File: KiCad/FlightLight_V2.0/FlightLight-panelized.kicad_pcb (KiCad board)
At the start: 2 copper layers, 69 x 73 mm, 116 parts, among them J3 Conn_02x05_Odd_Even, SW1 AP, U2 ULN2003, U3 ESP-12F, U4 AMS1117-3.3

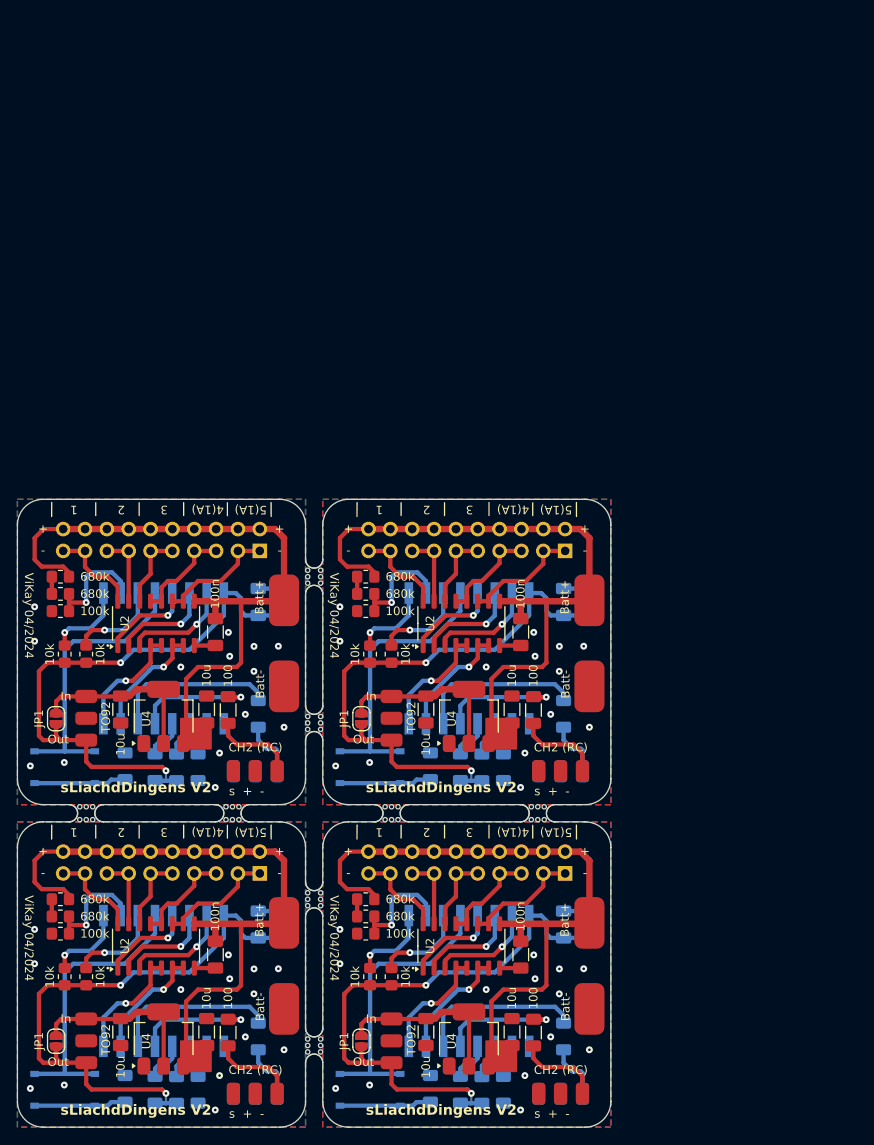
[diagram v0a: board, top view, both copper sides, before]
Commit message: new panelized
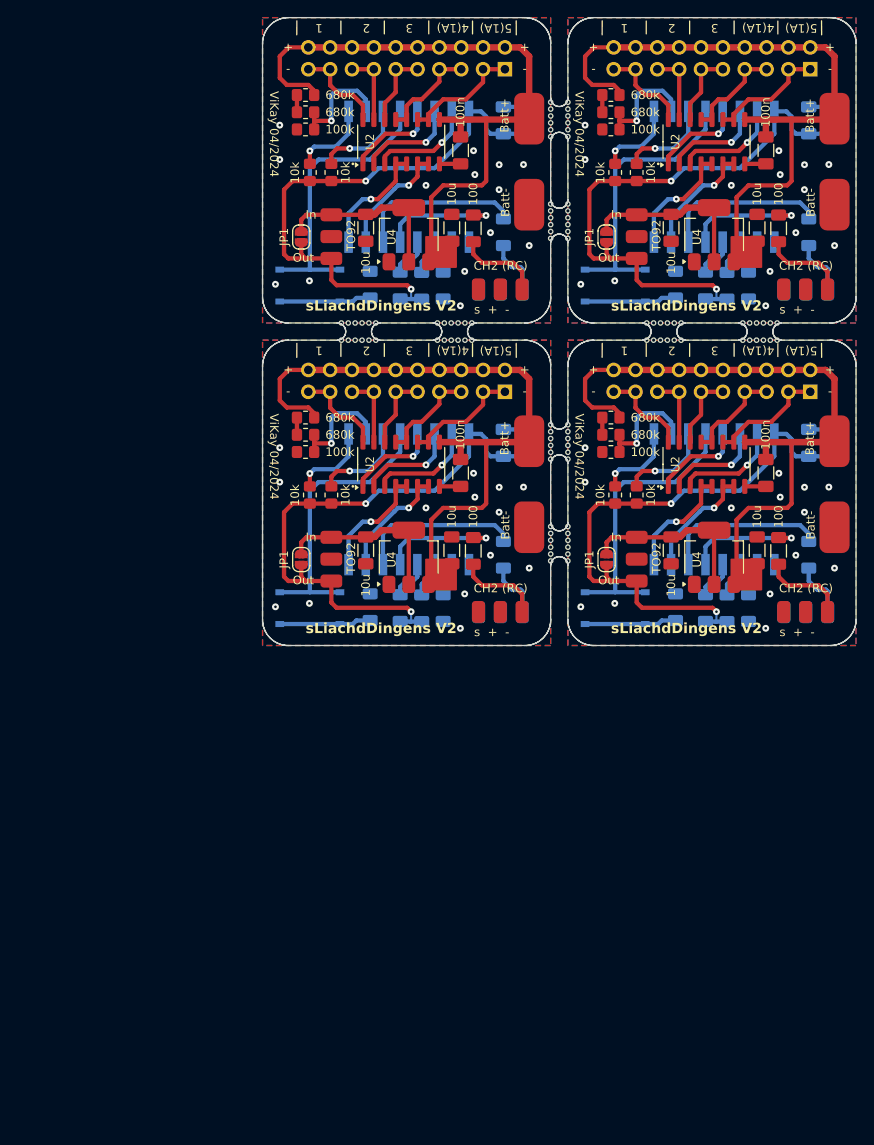
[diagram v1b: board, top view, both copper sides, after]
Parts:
- removed the Batt+1 at (152.0, 125.2)
- removed the Batt+1 at (116.5, 87.8)
- removed the Batt+1 at (116.5, 125.2)
- removed the Batt+1 at (152.0, 87.8)
- removed the Batt-1 at (116.5, 135.2)
- removed the Batt-1 at (116.5, 97.8)
- removed the Batt-1 at (152.0, 97.8)
- removed the Batt-1 at (152.0, 135.2)
- removed the C2 at (144.0, 91.4)
- removed the C2 at (144.0, 128.9)
- removed the C2 at (108.5, 128.9)
- removed the C2 at (108.5, 91.4)
- removed the C3 at (143.0, 100.4)
- removed the C3 at (107.5, 137.9)
- removed the C3 at (107.5, 100.4)
- removed the C3 at (143.0, 137.9)
- removed the C4 at (97.5, 137.9)
- removed the C4 at (133.0, 137.9)
- removed the C4 at (97.5, 100.4)
- removed the C4 at (133.0, 100.4)
- removed the C5 at (113.5, 87.9)
- removed the C5 at (149.0, 125.4)
- removed the C5 at (149.0, 87.9)
- removed the C5 at (113.5, 125.4)
- removed the C6 at (116.0, 87.9)
- removed the C6 at (151.5, 125.4)
- removed the C6 at (116.0, 125.4)
- removed the C6 at (151.5, 87.9)
- removed the CH1(RC)1 at (151.2, 107.6)
- removed the CH1(RC)1 at (115.7, 107.6)
- removed the CH1(RC)1 at (115.7, 145.1)
- removed the CH1(RC)1 at (151.2, 145.1)
- removed the CH2(RC)1 at (115.7, 145.1)
- removed the CH2(RC)1 at (115.7, 107.6)
- removed the CH2(RC)1 at (151.2, 145.1)
- removed the CH2(RC)1 at (151.2, 107.6)
- removed the J3 at (113.7, 82.0)
- removed the J3 at (149.2, 119.5)
- removed the J3 at (149.2, 82.0)
- removed the J3 at (113.7, 119.5)
- removed the JP1 at (125.5, 101.5)
- removed the JP1 at (90.0, 139.0)
- removed the JP1 at (90.0, 101.5)
- removed the JP1 at (125.5, 139.0)
- removed the R1 at (129.0, 94.0)
- removed the R1 at (129.0, 131.5)
- removed the R1 at (93.5, 131.5)
- removed the R1 at (93.5, 94.0)
- removed the R10 at (90.5, 124.5)
- removed the R10 at (126.0, 124.5)
- removed the R10 at (90.5, 87.0)
- removed the R10 at (126.0, 87.0)
- removed the R11 at (90.5, 122.5)
- removed the R11 at (126.0, 85.0)
- removed the R11 at (90.5, 85.0)
- removed the R11 at (126.0, 122.5)
- removed the R2 at (133.5, 144.5)
- removed the R2 at (98.0, 144.5)
- removed the R2 at (98.0, 107.0)
- removed the R2 at (133.5, 107.0)
- removed the R3 at (126.5, 94.0)
- removed the R3 at (91.0, 94.0)
- removed the R3 at (91.0, 131.5)
- removed the R3 at (126.5, 131.5)
- removed the R4 at (137.0, 144.6)
- removed the R4 at (101.5, 144.6)
- removed the R4 at (137.0, 107.1)
- removed the R4 at (101.5, 107.1)
- removed the R5 at (104.0, 144.7)
- removed the R5 at (104.0, 107.2)
- removed the R5 at (139.5, 144.7)
- removed the R5 at (139.5, 107.2)
- removed the R6 at (106.5, 144.7)
- removed the R6 at (142.0, 144.7)
- removed the R6 at (142.0, 107.2)
- removed the R6 at (106.5, 107.2)
- removed the R7 at (149.0, 138.4)
- removed the R7 at (113.5, 101.0)
- removed the R7 at (149.0, 101.0)
- removed the R7 at (113.5, 138.4)
- removed the R8 at (145.5, 100.5)
- removed the R8 at (110.0, 138.0)
- removed the R8 at (110.0, 100.5)
- removed the R8 at (145.5, 138.0)
- removed the R9 at (90.5, 89.0)
- removed the R9 at (126.0, 89.0)
- removed the R9 at (90.5, 126.5)
- removed the R9 at (126.0, 126.5)
- removed the SW1 at (91.0, 144.7)
- removed the SW1 at (91.0, 107.2)
- removed the SW1 at (126.5, 107.2)
- removed the SW1 at (126.5, 144.7)
- removed the TO92 at (129.0, 136.4)
- removed the TO92 at (93.5, 98.9)
- removed the TO92 at (129.0, 98.9)
- removed the TO92 at (93.5, 136.4)
- removed the U2 at (137.1, 127.9)
- removed the U2 at (101.6, 90.4)
- removed the U2 at (137.1, 90.4)
- removed the U2 at (101.6, 127.9)
- removed the U3 at (134.5, 94.5)
- removed the U3 at (99.0, 132.0)
- removed the U3 at (134.5, 132.0)
- removed the U3 at (99.0, 94.5)
- removed the U4 at (138.0, 101.2)
- removed the U4 at (138.0, 138.7)
- removed the U4 at (102.5, 101.2)
- removed the U4 at (102.5, 138.7)
- removed mouse-bite-2mm-slot (x8): VAL**, Panelization:mouse-bite-2mm-slot
- added Batt+1: Batt+, ViKay:Conn_01x01_2.54_big, F.Cu at (145.0, 69.2)
- added Batt+1: Batt+, ViKay:Conn_01x01_2.54_big, F.Cu at (180.5, 69.2)
- added Batt+1: Batt+, ViKay:Conn_01x01_2.54_big, F.Cu at (180.5, 31.8)
- added Batt+1: Batt+, ViKay:Conn_01x01_2.54_big, F.Cu at (145.0, 31.8)
- added Batt-1: Batt-, ViKay:Conn_01x01_2.54_big, F.Cu at (180.5, 79.2)
- added Batt-1: Batt-, ViKay:Conn_01x01_2.54_big, F.Cu at (145.0, 79.2)
- added Batt-1: Batt-, ViKay:Conn_01x01_2.54_big, F.Cu at (145.0, 41.8)
- added Batt-1: Batt-, ViKay:Conn_01x01_2.54_big, F.Cu at (180.5, 41.8)
- added C2: 100n, Capacitor_SMD:C_1206_3216Metric_Pad1.33x1.80mm_HandSolder, F.Cu at (137.0, 72.9)
- added C2: 100n, Capacitor_SMD:C_1206_3216Metric_Pad1.33x1.80mm_HandSolder, F.Cu at (137.0, 35.4)
- added C2: 100n, Capacitor_SMD:C_1206_3216Metric_Pad1.33x1.80mm_HandSolder, F.Cu at (172.5, 72.9)
- added C2: 100n, Capacitor_SMD:C_1206_3216Metric_Pad1.33x1.80mm_HandSolder, F.Cu at (172.5, 35.4)
- added C3: 10u, Capacitor_SMD:C_1206_3216Metric_Pad1.33x1.80mm_HandSolder, F.Cu at (171.5, 44.4)
- added C3: 10u, Capacitor_SMD:C_1206_3216Metric_Pad1.33x1.80mm_HandSolder, F.Cu at (171.5, 81.9)
- added C3: 10u, Capacitor_SMD:C_1206_3216Metric_Pad1.33x1.80mm_HandSolder, F.Cu at (136.0, 44.4)
- added C3: 10u, Capacitor_SMD:C_1206_3216Metric_Pad1.33x1.80mm_HandSolder, F.Cu at (136.0, 81.9)
- added C4: 10u, Capacitor_SMD:C_1206_3216Metric_Pad1.33x1.80mm_HandSolder, F.Cu at (161.5, 81.9)
- added C4: 10u, Capacitor_SMD:C_1206_3216Metric_Pad1.33x1.80mm_HandSolder, F.Cu at (126.0, 44.4)
- added C4: 10u, Capacitor_SMD:C_1206_3216Metric_Pad1.33x1.80mm_HandSolder, F.Cu at (161.5, 44.4)
- added C4: 10u, Capacitor_SMD:C_1206_3216Metric_Pad1.33x1.80mm_HandSolder, F.Cu at (126.0, 81.9)
- added C5: 100n, Capacitor_SMD:C_1206_3216Metric_Pad1.33x1.80mm_HandSolder, B.Cu at (142.0, 31.9)
- added C5: 100n, Capacitor_SMD:C_1206_3216Metric_Pad1.33x1.80mm_HandSolder, B.Cu at (142.0, 69.4)
- added C5: 100n, Capacitor_SMD:C_1206_3216Metric_Pad1.33x1.80mm_HandSolder, B.Cu at (177.5, 69.4)
- added C5: 100n, Capacitor_SMD:C_1206_3216Metric_Pad1.33x1.80mm_HandSolder, B.Cu at (177.5, 31.9)
- added C6: 10u, Capacitor_SMD:C_1206_3216Metric_Pad1.33x1.80mm_HandSolder, B.Cu at (144.5, 69.4)
- added C6: 10u, Capacitor_SMD:C_1206_3216Metric_Pad1.33x1.80mm_HandSolder, B.Cu at (180.0, 69.4)
- added C6: 10u, Capacitor_SMD:C_1206_3216Metric_Pad1.33x1.80mm_HandSolder, B.Cu at (180.0, 31.9)
- added C6: 10u, Capacitor_SMD:C_1206_3216Metric_Pad1.33x1.80mm_HandSolder, B.Cu at (144.5, 31.9)
- added CH1(RC)1: CH1 (RC), ViKay:Conn_01x03_2.54_small, B.Cu at (144.2, 89.1)
- added CH1(RC)1: CH1 (RC), ViKay:Conn_01x03_2.54_small, B.Cu at (179.7, 89.1)
- added CH1(RC)1: CH1 (RC), ViKay:Conn_01x03_2.54_small, B.Cu at (179.7, 51.6)
- added CH1(RC)1: CH1 (RC), ViKay:Conn_01x03_2.54_small, B.Cu at (144.2, 51.6)
- added CH2(RC)1: CH2 (RC) LowPower, ViKay:Conn_01x03_2.54_small, F.Cu at (179.7, 51.6)
- added CH2(RC)1: CH2 (RC) LowPower, ViKay:Conn_01x03_2.54_small, F.Cu at (144.2, 89.1)
- added CH2(RC)1: CH2 (RC) LowPower, ViKay:Conn_01x03_2.54_small, F.Cu at (144.2, 51.6)
- added CH2(RC)1: CH2 (RC) LowPower, ViKay:Conn_01x03_2.54_small, F.Cu at (179.7, 89.1)
- added J3: Conn_02x05_Odd_Even, Connector_PinHeader_2.54mm:PinHeader_2x10_P2.54mm_Vertical, B.Cu at (177.7, 63.5)
- added J3: Conn_02x05_Odd_Even, Connector_PinHeader_2.54mm:PinHeader_2x10_P2.54mm_Vertical, B.Cu at (177.7, 26.0)
- added J3: Conn_02x05_Odd_Even, Connector_PinHeader_2.54mm:PinHeader_2x10_P2.54mm_Vertical, B.Cu at (142.2, 26.0)
- added J3: Conn_02x05_Odd_Even, Connector_PinHeader_2.54mm:PinHeader_2x10_P2.54mm_Vertical, B.Cu at (142.2, 63.5)
- added JP1: kein Supervisor, Jumper:SolderJumper-2_P1.3mm_Open_RoundedPad1.0x1.5mm, F.Cu at (118.5, 45.5)
- added JP1: kein Supervisor, Jumper:SolderJumper-2_P1.3mm_Open_RoundedPad1.0x1.5mm, F.Cu at (118.5, 83.0)
- added JP1: kein Supervisor, Jumper:SolderJumper-2_P1.3mm_Open_RoundedPad1.0x1.5mm, F.Cu at (154.0, 83.0)
- added JP1: kein Supervisor, Jumper:SolderJumper-2_P1.3mm_Open_RoundedPad1.0x1.5mm, F.Cu at (154.0, 45.5)
- added KiKit_MB_10_1: NPTH, NPTH, F.Cu at (147.5, 79.2)
- added KiKit_MB_10_2: NPTH, NPTH, F.Cu at (147.5, 80.0)
- added KiKit_MB_10_3: NPTH, NPTH, F.Cu at (147.5, 80.8)
- added KiKit_MB_10_4: NPTH, NPTH, F.Cu at (147.5, 81.6)
- added KiKit_MB_10_5: NPTH, NPTH, F.Cu at (147.5, 82.4)
- added KiKit_MB_10_6: NPTH, NPTH, F.Cu at (147.5, 83.2)
- added KiKit_MB_11_1: NPTH, NPTH, F.Cu at (123.2, 57.5)
- added KiKit_MB_11_2: NPTH, NPTH, F.Cu at (124.0, 57.5)
- added KiKit_MB_11_3: NPTH, NPTH, F.Cu at (124.8, 57.5)
- added KiKit_MB_11_4: NPTH, NPTH, F.Cu at (125.6, 57.5)
- added KiKit_MB_11_5: NPTH, NPTH, F.Cu at (126.4, 57.5)
- added KiKit_MB_11_6: NPTH, NPTH, F.Cu at (127.2, 57.5)
- added KiKit_MB_12_1: NPTH, NPTH, F.Cu at (134.3, 57.5)
- added KiKit_MB_12_2: NPTH, NPTH, F.Cu at (135.1, 57.5)
- added KiKit_MB_12_3: NPTH, NPTH, F.Cu at (135.9, 57.5)
- added KiKit_MB_12_4: NPTH, NPTH, F.Cu at (136.7, 57.5)
- added KiKit_MB_12_5: NPTH, NPTH, F.Cu at (137.5, 57.5)
- added KiKit_MB_12_6: NPTH, NPTH, F.Cu at (138.3, 57.5)
- added KiKit_MB_13_1: NPTH, NPTH, F.Cu at (149.5, 71.3)
- added KiKit_MB_13_2: NPTH, NPTH, F.Cu at (149.5, 70.5)
- added KiKit_MB_13_3: NPTH, NPTH, F.Cu at (149.5, 69.7)
- added KiKit_MB_13_4: NPTH, NPTH, F.Cu at (149.5, 68.9)
- added KiKit_MB_13_5: NPTH, NPTH, F.Cu at (149.5, 68.1)
- added KiKit_MB_13_6: NPTH, NPTH, F.Cu at (149.5, 67.3)
- added KiKit_MB_14_1: NPTH, NPTH, F.Cu at (149.5, 83.2)
- added KiKit_MB_14_2: NPTH, NPTH, F.Cu at (149.5, 82.4)
- added KiKit_MB_14_3: NPTH, NPTH, F.Cu at (149.5, 81.6)
- added KiKit_MB_14_4: NPTH, NPTH, F.Cu at (149.5, 80.8)
- added KiKit_MB_14_5: NPTH, NPTH, F.Cu at (149.5, 80.0)
- added KiKit_MB_14_6: NPTH, NPTH, F.Cu at (149.5, 79.2)
- added KiKit_MB_15_1: NPTH, NPTH, F.Cu at (158.7, 57.5)
- added KiKit_MB_15_2: NPTH, NPTH, F.Cu at (159.5, 57.5)
- added KiKit_MB_15_3: NPTH, NPTH, F.Cu at (160.3, 57.5)
- added KiKit_MB_15_4: NPTH, NPTH, F.Cu at (161.1, 57.5)
- added KiKit_MB_15_5: NPTH, NPTH, F.Cu at (161.9, 57.5)
- added KiKit_MB_15_6: NPTH, NPTH, F.Cu at (162.7, 57.5)
- added KiKit_MB_16_1: NPTH, NPTH, F.Cu at (169.8, 57.5)
- added KiKit_MB_16_2: NPTH, NPTH, F.Cu at (170.6, 57.5)
- added KiKit_MB_16_3: NPTH, NPTH, F.Cu at (171.4, 57.5)
- added KiKit_MB_16_4: NPTH, NPTH, F.Cu at (172.2, 57.5)
- added KiKit_MB_16_5: NPTH, NPTH, F.Cu at (173.0, 57.5)
- added KiKit_MB_16_6: NPTH, NPTH, F.Cu at (173.8, 57.5)
- added KiKit_MB_1_1: NPTH, NPTH, F.Cu at (147.5, 29.8)
- added KiKit_MB_1_2: NPTH, NPTH, F.Cu at (147.5, 30.6)
- added KiKit_MB_1_3: NPTH, NPTH, F.Cu at (147.5, 31.4)
- added KiKit_MB_1_4: NPTH, NPTH, F.Cu at (147.5, 32.2)
- added KiKit_MB_1_5: NPTH, NPTH, F.Cu at (147.5, 33.0)
- added KiKit_MB_1_6: NPTH, NPTH, F.Cu at (147.5, 33.8)
- added KiKit_MB_2_1: NPTH, NPTH, F.Cu at (147.5, 41.7)
- added KiKit_MB_2_2: NPTH, NPTH, F.Cu at (147.5, 42.5)
- added KiKit_MB_2_3: NPTH, NPTH, F.Cu at (147.5, 43.3)
- added KiKit_MB_2_4: NPTH, NPTH, F.Cu at (147.5, 44.1)
- added KiKit_MB_2_5: NPTH, NPTH, F.Cu at (147.5, 44.9)
- added KiKit_MB_2_6: NPTH, NPTH, F.Cu at (147.5, 45.7)
- added KiKit_MB_3_1: NPTH, NPTH, F.Cu at (127.2, 55.5)
- added KiKit_MB_3_2: NPTH, NPTH, F.Cu at (126.4, 55.5)
- added KiKit_MB_3_3: NPTH, NPTH, F.Cu at (125.6, 55.5)
- added KiKit_MB_3_4: NPTH, NPTH, F.Cu at (124.8, 55.5)
- added KiKit_MB_3_5: NPTH, NPTH, F.Cu at (124.0, 55.5)
- added KiKit_MB_3_6: NPTH, NPTH, F.Cu at (123.2, 55.5)
- added KiKit_MB_4_1: NPTH, NPTH, F.Cu at (138.3, 55.5)
- added KiKit_MB_4_2: NPTH, NPTH, F.Cu at (137.5, 55.5)
- added KiKit_MB_4_3: NPTH, NPTH, F.Cu at (136.7, 55.5)
- added KiKit_MB_4_4: NPTH, NPTH, F.Cu at (135.9, 55.5)
- added KiKit_MB_4_5: NPTH, NPTH, F.Cu at (135.1, 55.5)
- added KiKit_MB_4_6: NPTH, NPTH, F.Cu at (134.3, 55.5)
- added KiKit_MB_5_1: NPTH, NPTH, F.Cu at (149.5, 33.8)
- added KiKit_MB_5_2: NPTH, NPTH, F.Cu at (149.5, 33.0)
- added KiKit_MB_5_3: NPTH, NPTH, F.Cu at (149.5, 32.2)
- added KiKit_MB_5_4: NPTH, NPTH, F.Cu at (149.5, 31.4)
- added KiKit_MB_5_5: NPTH, NPTH, F.Cu at (149.5, 30.6)
- added KiKit_MB_5_6: NPTH, NPTH, F.Cu at (149.5, 29.8)
- added KiKit_MB_6_1: NPTH, NPTH, F.Cu at (149.5, 45.7)
- added KiKit_MB_6_2: NPTH, NPTH, F.Cu at (149.5, 44.9)
- added KiKit_MB_6_3: NPTH, NPTH, F.Cu at (149.5, 44.1)
- added KiKit_MB_6_4: NPTH, NPTH, F.Cu at (149.5, 43.3)
- added KiKit_MB_6_5: NPTH, NPTH, F.Cu at (149.5, 42.5)
- added KiKit_MB_6_6: NPTH, NPTH, F.Cu at (149.5, 41.7)
- added KiKit_MB_7_1: NPTH, NPTH, F.Cu at (162.7, 55.5)
- added KiKit_MB_7_2: NPTH, NPTH, F.Cu at (161.9, 55.5)
- added KiKit_MB_7_3: NPTH, NPTH, F.Cu at (161.1, 55.5)
- added KiKit_MB_7_4: NPTH, NPTH, F.Cu at (160.3, 55.5)
- added KiKit_MB_7_5: NPTH, NPTH, F.Cu at (159.5, 55.5)
- added KiKit_MB_7_6: NPTH, NPTH, F.Cu at (158.7, 55.5)
- added KiKit_MB_8_1: NPTH, NPTH, F.Cu at (173.8, 55.5)
- added KiKit_MB_8_2: NPTH, NPTH, F.Cu at (173.0, 55.5)
- added KiKit_MB_8_3: NPTH, NPTH, F.Cu at (172.2, 55.5)
- added KiKit_MB_8_4: NPTH, NPTH, F.Cu at (171.4, 55.5)
- added KiKit_MB_8_5: NPTH, NPTH, F.Cu at (170.6, 55.5)
- added KiKit_MB_8_6: NPTH, NPTH, F.Cu at (169.8, 55.5)
- added KiKit_MB_9_1: NPTH, NPTH, F.Cu at (147.5, 67.3)
- added KiKit_MB_9_2: NPTH, NPTH, F.Cu at (147.5, 68.1)
- added KiKit_MB_9_3: NPTH, NPTH, F.Cu at (147.5, 68.9)
- added KiKit_MB_9_4: NPTH, NPTH, F.Cu at (147.5, 69.7)
- added KiKit_MB_9_5: NPTH, NPTH, F.Cu at (147.5, 70.5)
- added KiKit_MB_9_6: NPTH, NPTH, F.Cu at (147.5, 71.3)
- added R1: 10k, Resistor_SMD:R_0805_2012Metric_Pad1.20x1.40mm_HandSolder, F.Cu at (157.5, 38.0)
- added R1: 10k, Resistor_SMD:R_0805_2012Metric_Pad1.20x1.40mm_HandSolder, F.Cu at (157.5, 75.5)
- added R1: 10k, Resistor_SMD:R_0805_2012Metric_Pad1.20x1.40mm_HandSolder, F.Cu at (122.0, 75.5)
- added R1: 10k, Resistor_SMD:R_0805_2012Metric_Pad1.20x1.40mm_HandSolder, F.Cu at (122.0, 38.0)
- added R10: 680k, Resistor_SMD:R_0805_2012Metric_Pad1.20x1.40mm_HandSolder, F.Cu at (154.5, 31.0)
- added R10: 680k, Resistor_SMD:R_0805_2012Metric_Pad1.20x1.40mm_HandSolder, F.Cu at (154.5, 68.5)
- added R10: 680k, Resistor_SMD:R_0805_2012Metric_Pad1.20x1.40mm_HandSolder, F.Cu at (119.0, 68.5)
- added R10: 680k, Resistor_SMD:R_0805_2012Metric_Pad1.20x1.40mm_HandSolder, F.Cu at (119.0, 31.0)
- added R11: 680k, Resistor_SMD:R_0805_2012Metric_Pad1.20x1.40mm_HandSolder, F.Cu at (154.5, 29.0)
- added R11: 680k, Resistor_SMD:R_0805_2012Metric_Pad1.20x1.40mm_HandSolder, F.Cu at (119.0, 29.0)
- added R11: 680k, Resistor_SMD:R_0805_2012Metric_Pad1.20x1.40mm_HandSolder, F.Cu at (154.5, 66.5)
- added R11: 680k, Resistor_SMD:R_0805_2012Metric_Pad1.20x1.40mm_HandSolder, F.Cu at (119.0, 66.5)
- added R2: 10k, Resistor_SMD:R_1206_3216Metric_Pad1.30x1.75mm_HandSolder, B.Cu at (126.5, 51.0)
- added R2: 10k, Resistor_SMD:R_1206_3216Metric_Pad1.30x1.75mm_HandSolder, B.Cu at (126.5, 88.5)
- added R2: 10k, Resistor_SMD:R_1206_3216Metric_Pad1.30x1.75mm_HandSolder, B.Cu at (162.0, 88.5)
- added R2: 10k, Resistor_SMD:R_1206_3216Metric_Pad1.30x1.75mm_HandSolder, B.Cu at (162.0, 51.0)
- added R3: 10k, Resistor_SMD:R_0805_2012Metric_Pad1.20x1.40mm_HandSolder, F.Cu at (155.0, 75.5)
- added R3: 10k, Resistor_SMD:R_0805_2012Metric_Pad1.20x1.40mm_HandSolder, F.Cu at (119.5, 38.0)
- added R3: 10k, Resistor_SMD:R_0805_2012Metric_Pad1.20x1.40mm_HandSolder, F.Cu at (119.5, 75.5)
- added R3: 10k, Resistor_SMD:R_0805_2012Metric_Pad1.20x1.40mm_HandSolder, F.Cu at (155.0, 38.0)
- added R4: 10k, Resistor_SMD:R_1206_3216Metric_Pad1.30x1.75mm_HandSolder, B.Cu at (130.0, 51.1)
- added R4: 10k, Resistor_SMD:R_1206_3216Metric_Pad1.30x1.75mm_HandSolder, B.Cu at (130.0, 88.6)
- added R4: 10k, Resistor_SMD:R_1206_3216Metric_Pad1.30x1.75mm_HandSolder, B.Cu at (165.5, 88.6)
- added R4: 10k, Resistor_SMD:R_1206_3216Metric_Pad1.30x1.75mm_HandSolder, B.Cu at (165.5, 51.1)
- added R5: 10k, Resistor_SMD:R_1206_3216Metric_Pad1.30x1.75mm_HandSolder, B.Cu at (132.5, 88.7)
- added R5: 10k, Resistor_SMD:R_1206_3216Metric_Pad1.30x1.75mm_HandSolder, B.Cu at (168.0, 51.2)
- added R5: 10k, Resistor_SMD:R_1206_3216Metric_Pad1.30x1.75mm_HandSolder, B.Cu at (168.0, 88.7)
- added R5: 10k, Resistor_SMD:R_1206_3216Metric_Pad1.30x1.75mm_HandSolder, B.Cu at (132.5, 51.2)
- added R6: 10k, Resistor_SMD:R_1206_3216Metric_Pad1.30x1.75mm_HandSolder, B.Cu at (170.5, 51.1)
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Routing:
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- added copper zone on B.Cu, net Board_0--BATT
- added copper zone on F.Cu, net Board_0--BATT
- added copper zone on B.Cu, net Board_1--BATT
- added copper zone on F.Cu, net Board_1--BATT
- added copper zone on B.Cu, net Board_2--BATT
- added copper zone on F.Cu, net Board_2--BATT
- added copper zone on B.Cu, net Board_3--BATT
- added copper zone on F.Cu, net Board_3--BATT
- removed copper zone on B.Cu, net -BATT
- removed copper zone on F.Cu, net -BATT
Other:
- outline, holes or cut-outs redrawn

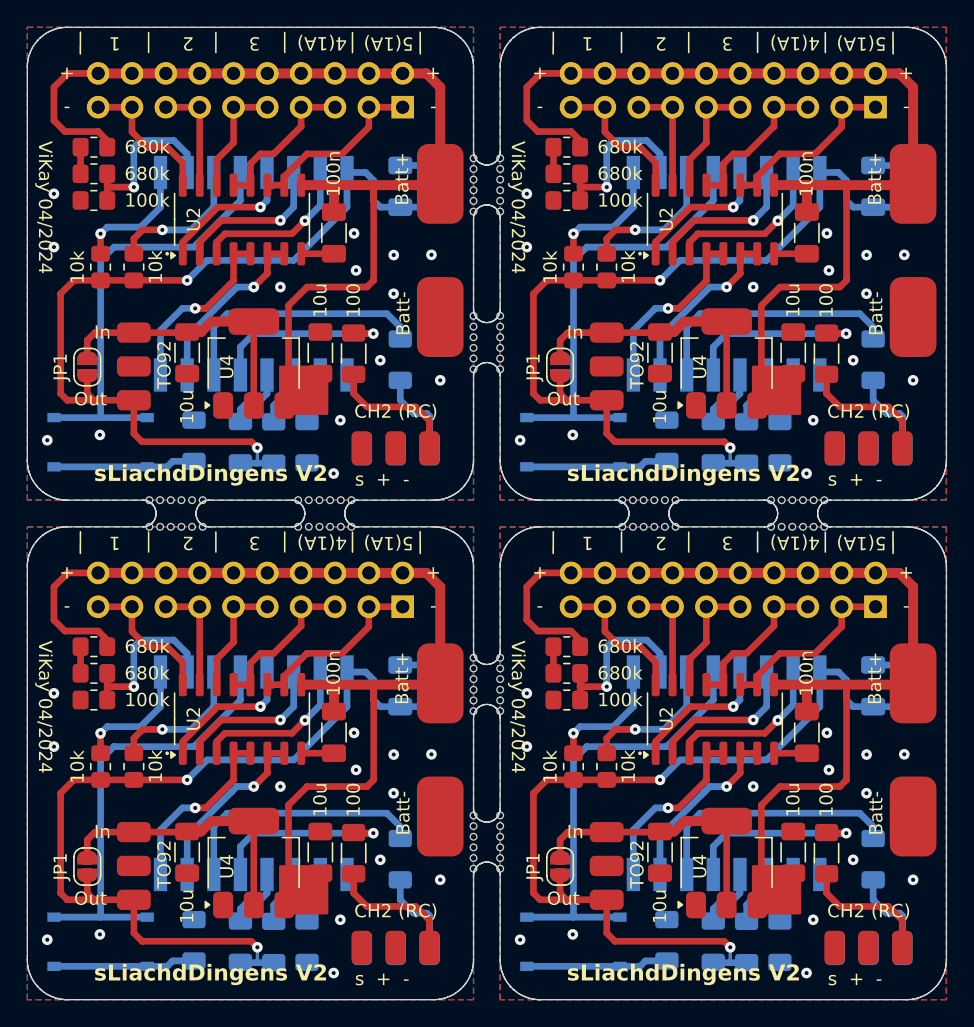
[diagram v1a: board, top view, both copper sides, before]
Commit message: PCB V2.1
kleine Fixes
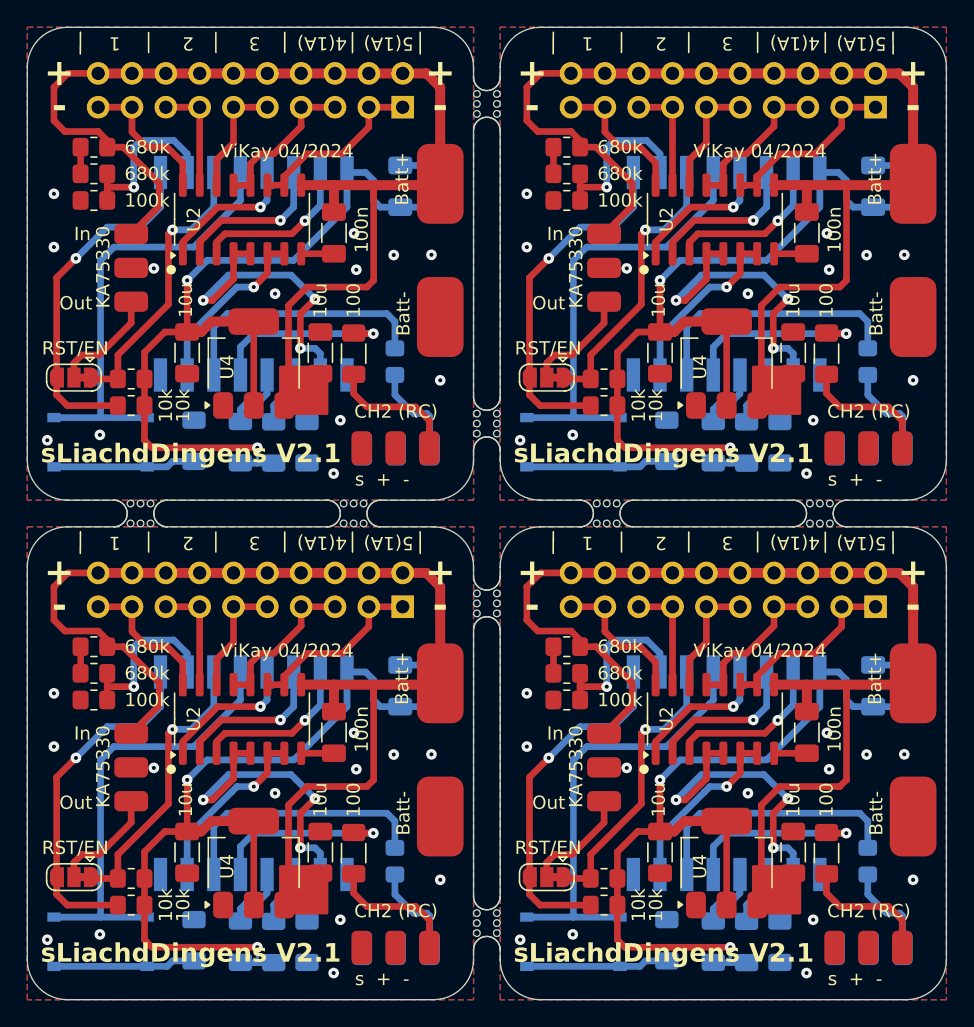
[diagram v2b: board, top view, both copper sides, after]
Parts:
- removed the JP1 at (118.5, 45.5)
- removed the JP1 at (118.5, 83.0)
- removed the JP1 at (154.0, 83.0)
- removed the JP1 at (154.0, 45.5)
- removed KiKit_MB_10_1, KiKit_MB_10_2, KiKit_MB_10_3, KiKit_MB_10_4, KiKit_MB_10_5, KiKit_MB_10_6, KiKit_MB_11_1, KiKit_MB_11_2, KiKit_MB_11_3, KiKit_MB_11_4, KiKit_MB_11_5, KiKit_MB_11_6, KiKit_MB_12_1, KiKit_MB_12_2, KiKit_MB_12_3, KiKit_MB_12_4, KiKit_MB_12_5, KiKit_MB_12_6, KiKit_MB_13_1, KiKit_MB_13_2, KiKit_MB_13_3, KiKit_MB_13_4, KiKit_MB_13_5, KiKit_MB_13_6, KiKit_MB_14_1, KiKit_MB_14_2, KiKit_MB_14_3, KiKit_MB_14_4, KiKit_MB_14_5, KiKit_MB_14_6, KiKit_MB_15_1, KiKit_MB_15_2, KiKit_MB_15_3, KiKit_MB_15_4, KiKit_MB_15_5, KiKit_MB_15_6, KiKit_MB_16_1, KiKit_MB_16_2, KiKit_MB_16_3, KiKit_MB_16_4, KiKit_MB_16_5, KiKit_MB_16_6, KiKit_MB_1_1, KiKit_MB_1_2, KiKit_MB_1_3, KiKit_MB_1_4, KiKit_MB_1_5, KiKit_MB_1_6, KiKit_MB_2_1, KiKit_MB_2_2, KiKit_MB_2_3, KiKit_MB_2_4, KiKit_MB_2_5, KiKit_MB_2_6, KiKit_MB_3_1, KiKit_MB_3_2, KiKit_MB_3_3, KiKit_MB_3_4, KiKit_MB_3_5, KiKit_MB_3_6, KiKit_MB_4_1, KiKit_MB_4_2, KiKit_MB_4_3, KiKit_MB_4_4, KiKit_MB_4_5, KiKit_MB_4_6, KiKit_MB_5_1, KiKit_MB_5_2, KiKit_MB_5_3, KiKit_MB_5_4, KiKit_MB_5_5, KiKit_MB_5_6, KiKit_MB_6_1, KiKit_MB_6_2, KiKit_MB_6_3, KiKit_MB_6_4, KiKit_MB_6_5, KiKit_MB_6_6, KiKit_MB_7_1, KiKit_MB_7_2, KiKit_MB_7_3, KiKit_MB_7_4, KiKit_MB_7_5, KiKit_MB_7_6, KiKit_MB_8_1, KiKit_MB_8_2, KiKit_MB_8_3, KiKit_MB_8_4, KiKit_MB_8_5, KiKit_MB_8_6, KiKit_MB_9_1, KiKit_MB_9_2, KiKit_MB_9_3, KiKit_MB_9_4, KiKit_MB_9_5, KiKit_MB_9_6: NPTH, NPTH
- removed the R1 at (157.5, 38.0)
- removed the R1 at (157.5, 75.5)
- removed the R1 at (122.0, 75.5)
- removed the R1 at (122.0, 38.0)
- removed the R3 at (155.0, 75.5)
- removed the R3 at (119.5, 38.0)
- removed the R3 at (119.5, 75.5)
- removed the R3 at (155.0, 38.0)
- removed the R7 at (142.0, 82.5)
- removed the R7 at (142.0, 45.0)
- removed the R7 at (177.5, 45.0)
- removed the R7 at (177.5, 82.5)
- removed the TO92 at (157.5, 42.9)
- removed the TO92 at (157.5, 80.4)
- removed the TO92 at (122.0, 42.9)
- removed the TO92 at (122.0, 80.4)
- added JP1: RST/EN, Jumper:SolderJumper-3_P1.3mm_Bridged12_RoundedPad1.0x1.5mm, F.Cu at (153.0, 83.8)
- added JP1: RST/EN, Jumper:SolderJumper-3_P1.3mm_Bridged12_RoundedPad1.0x1.5mm, F.Cu at (153.0, 46.3)
- added JP1: RST/EN, Jumper:SolderJumper-3_P1.3mm_Bridged12_RoundedPad1.0x1.5mm, F.Cu at (117.5, 83.8)
- added JP1: RST/EN, Jumper:SolderJumper-3_P1.3mm_Bridged12_RoundedPad1.0x1.5mm, F.Cu at (117.5, 46.3)
- added R1: 10k, Resistor_SMD:R_0805_2012Metric_Pad1.20x1.40mm_HandSolder, F.Cu at (157.3, 46.4)
- added R1: 10k, Resistor_SMD:R_0805_2012Metric_Pad1.20x1.40mm_HandSolder, F.Cu at (121.8, 83.9)
- added R1: 10k, Resistor_SMD:R_0805_2012Metric_Pad1.20x1.40mm_HandSolder, F.Cu at (157.3, 83.9)
- added R1: 10k, Resistor_SMD:R_0805_2012Metric_Pad1.20x1.40mm_HandSolder, F.Cu at (121.8, 46.4)
- added R3: 10k, Resistor_SMD:R_0805_2012Metric_Pad1.20x1.40mm_HandSolder, F.Cu at (121.8, 48.4)
- added R3: 10k, Resistor_SMD:R_0805_2012Metric_Pad1.20x1.40mm_HandSolder, F.Cu at (157.3, 85.9)
- added R3: 10k, Resistor_SMD:R_0805_2012Metric_Pad1.20x1.40mm_HandSolder, F.Cu at (157.3, 48.4)
- added R3: 10k, Resistor_SMD:R_0805_2012Metric_Pad1.20x1.40mm_HandSolder, F.Cu at (121.8, 85.9)
- added R7: 100, Resistor_SMD:R_0805_2012Metric_Pad1.20x1.40mm_HandSolder, B.Cu at (177.1, 45.1)
- added R7: 100, Resistor_SMD:R_0805_2012Metric_Pad1.20x1.40mm_HandSolder, B.Cu at (141.6, 82.6)
- added R7: 100, Resistor_SMD:R_0805_2012Metric_Pad1.20x1.40mm_HandSolder, B.Cu at (177.1, 82.6)
- added R7: 100, Resistor_SMD:R_0805_2012Metric_Pad1.20x1.40mm_HandSolder, B.Cu at (141.6, 45.1)
- added TO92: KA75330, ViKay:Conn_01x03_2.54_small, F.Cu at (121.8, 73.0)
- added TO92: KA75330, ViKay:Conn_01x03_2.54_small, F.Cu at (157.3, 73.0)
- added TO92: KA75330, ViKay:Conn_01x03_2.54_small, F.Cu at (121.8, 35.5)
- added TO92: KA75330, ViKay:Conn_01x03_2.54_small, F.Cu at (157.3, 35.5)
- added mouse-bite-2mm-slot: VAL**, Panelization:mouse-bite-2mm-slot, F.Cu at (148.5, 87.2)
- added mouse-bite-2mm-slot: VAL**, Panelization:mouse-bite-2mm-slot, F.Cu at (148.5, 63.2)
- added mouse-bite-2mm-slot: VAL**, Panelization:mouse-bite-2mm-slot, F.Cu at (148.5, 25.8)
- added mouse-bite-2mm-slot: VAL**, Panelization:mouse-bite-2mm-slot, F.Cu at (138.5, 56.5)
- added mouse-bite-2mm-slot: VAL**, Panelization:mouse-bite-2mm-slot, F.Cu at (157.5, 56.5)
- added mouse-bite-2mm-slot: VAL**, Panelization:mouse-bite-2mm-slot, F.Cu at (122.5, 56.5)
- added mouse-bite-2mm-slot: VAL**, Panelization:mouse-bite-2mm-slot, F.Cu at (173.5, 56.5)
- added mouse-bite-2mm-slot: VAL**, Panelization:mouse-bite-2mm-slot, F.Cu at (148.5, 49.8)
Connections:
- Batt+1 pad 1: Board_3-+BATT -> +BATT
- Batt+1 pad 1: Board_2-+BATT -> +BATT
- Batt+1 pad 1: Board_1-+BATT -> +BATT
- Batt+1 pad 1: Board_0-+BATT -> +BATT
- Batt-1 pad 1: Board_0--BATT -> -BATT
- Batt-1 pad 1: Board_2--BATT -> -BATT
- Batt-1 pad 1: Board_3--BATT -> -BATT
- Batt-1 pad 1: Board_1--BATT -> -BATT
- C2 pad 1: Board_3-+BATT -> +BATT
- C2 pad 2: Board_3--BATT -> -BATT
- C2 pad 1: Board_1-+BATT -> +BATT
- C2 pad 2: Board_1--BATT -> -BATT
- C2 pad 1: Board_2-+BATT -> +BATT
- C2 pad 2: Board_2--BATT -> -BATT
- C2 pad 1: Board_0-+BATT -> +BATT
- C2 pad 2: Board_0--BATT -> -BATT
- C3 pad 1: Board_3-+BATT -> +BATT
- C3 pad 2: Board_3--BATT -> -BATT
- C3 pad 1: Board_1-+BATT -> +BATT
- C3 pad 2: Board_1--BATT -> -BATT
- C3 pad 1: Board_2-+BATT -> +BATT
- C3 pad 2: Board_2--BATT -> -BATT
- C3 pad 1: Board_0-+BATT -> +BATT
- C3 pad 2: Board_0--BATT -> -BATT
- C4 pad 1: Board_2-Net-(JP1-A) -> 3,3V
- C4 pad 2: Board_2--BATT -> -BATT
- C4 pad 1: Board_0-Net-(JP1-A) -> 3,3V
- C4 pad 2: Board_0--BATT -> -BATT
- C4 pad 1: Board_1-Net-(JP1-A) -> 3,3V
- C4 pad 2: Board_1--BATT -> -BATT
- C4 pad 1: Board_3-Net-(JP1-A) -> 3,3V
- C4 pad 2: Board_3--BATT -> -BATT
- C5 pad 1: Board_1--BATT -> -BATT
- C5 pad 2: Board_1-3,3V -> 3,3V
- C5 pad 1: Board_3--BATT -> -BATT
- C5 pad 2: Board_3-3,3V -> 3,3V
- C5 pad 1: Board_2--BATT -> -BATT
- C5 pad 2: Board_2-3,3V -> 3,3V
- C5 pad 1: Board_0--BATT -> -BATT
- C5 pad 2: Board_0-3,3V -> 3,3V
- C6 pad 1: Board_2--BATT -> -BATT
- C6 pad 2: Board_2-3,3V -> 3,3V
- C6 pad 1: Board_3--BATT -> -BATT
- C6 pad 2: Board_3-3,3V -> 3,3V
- C6 pad 1: Board_1--BATT -> -BATT
- C6 pad 2: Board_1-3,3V -> 3,3V
- C6 pad 1: Board_0--BATT -> -BATT
- C6 pad 2: Board_0-3,3V -> 3,3V
- CH1(RC)1 pad 1: Board_1-/CH1 -> /CH1
- CH1(RC)1 pad 2: Board_1-unconnected-(CH1(RC)1-Pin_2-Pad2) -> unconnected-(CH1(RC)1-Pin_2-Pad2)
- CH1(RC)1 pad 3: Board_1--BATT -> -BATT
- CH1(RC)1 pad 1: Board_3-/CH1 -> /CH1
- CH1(RC)1 pad 2: Board_3-unconnected-(CH1(RC)1-Pin_2-Pad2) -> unconnected-(CH1(RC)1-Pin_2-Pad2)
- CH1(RC)1 pad 3: Board_3--BATT -> -BATT
- CH1(RC)1 pad 1: Board_0-/CH1 -> /CH1
- CH1(RC)1 pad 2: Board_0-unconnected-(CH1(RC)1-Pin_2-Pad2) -> unconnected-(CH1(RC)1-Pin_2-Pad2)
- CH1(RC)1 pad 3: Board_0--BATT -> -BATT
- CH1(RC)1 pad 1: Board_2-/CH1 -> /CH1
- CH1(RC)1 pad 2: Board_2-unconnected-(CH1(RC)1-Pin_2-Pad2) -> unconnected-(CH1(RC)1-Pin_2-Pad2)
- CH1(RC)1 pad 3: Board_2--BATT -> -BATT
- CH2(RC)1 pad 1: Board_3-/CH2 -> /CH2
- CH2(RC)1 pad 2: Board_3-unconnected-(CH2(RC)1-Pin_2-Pad2) -> unconnected-(CH2(RC)1-Pin_2-Pad2)
- CH2(RC)1 pad 3: Board_3--BATT -> -BATT
- CH2(RC)1 pad 1: Board_2-/CH2 -> /CH2
- CH2(RC)1 pad 2: Board_2-unconnected-(CH2(RC)1-Pin_2-Pad2) -> unconnected-(CH2(RC)1-Pin_2-Pad2)
- CH2(RC)1 pad 3: Board_2--BATT -> -BATT
- CH2(RC)1 pad 1: Board_0-/CH2 -> /CH2
- CH2(RC)1 pad 2: Board_0-unconnected-(CH2(RC)1-Pin_2-Pad2) -> unconnected-(CH2(RC)1-Pin_2-Pad2)
- CH2(RC)1 pad 3: Board_0--BATT -> -BATT
- CH2(RC)1 pad 1: Board_1-/CH2 -> /CH2
- CH2(RC)1 pad 2: Board_1-unconnected-(CH2(RC)1-Pin_2-Pad2) -> unconnected-(CH2(RC)1-Pin_2-Pad2)
- CH2(RC)1 pad 3: Board_1--BATT -> -BATT
- J3 pad 1: Board_3-Net-(J3-Pin_1) -> Net-(J3-Pin_1)
- J3 pad 10: Board_3-+BATT -> +BATT
- J3 pad 11: Board_3-Net-(J3-Pin_11) -> Net-(J3-Pin_11)
- J3 pad 12: Board_3-+BATT -> +BATT
- J3 pad 13: Board_3-Net-(J3-Pin_13) -> Net-(J3-Pin_13)
- J3 pad 14: Board_3-+BATT -> +BATT
- J3 pad 15: Board_3-Net-(J3-Pin_13) -> Net-(J3-Pin_13)
- J3 pad 16: Board_3-+BATT -> +BATT
- J3 pad 17: Board_3-Net-(J3-Pin_17) -> Net-(J3-Pin_17)
- J3 pad 18: Board_3-+BATT -> +BATT
- J3 pad 19: Board_3-Net-(J3-Pin_17) -> Net-(J3-Pin_17)
- J3 pad 2: Board_3-+BATT -> +BATT
- J3 pad 20: Board_3-+BATT -> +BATT
- J3 pad 3: Board_3-Net-(J3-Pin_1) -> Net-(J3-Pin_1)
- J3 pad 4: Board_3-+BATT -> +BATT
- J3 pad 5: Board_3-Net-(J3-Pin_5) -> Net-(J3-Pin_5)
- J3 pad 6: Board_3-+BATT -> +BATT
- J3 pad 7: Board_3-Net-(J3-Pin_5) -> Net-(J3-Pin_5)
- J3 pad 8: Board_3-+BATT -> +BATT
- J3 pad 9: Board_3-Net-(J3-Pin_11) -> Net-(J3-Pin_11)
- J3 pad 1: Board_2-Net-(J3-Pin_1) -> Net-(J3-Pin_1)
- J3 pad 10: Board_2-+BATT -> +BATT
- J3 pad 11: Board_2-Net-(J3-Pin_11) -> Net-(J3-Pin_11)
- J3 pad 12: Board_2-+BATT -> +BATT
- J3 pad 13: Board_2-Net-(J3-Pin_13) -> Net-(J3-Pin_13)
- J3 pad 14: Board_2-+BATT -> +BATT
- J3 pad 15: Board_2-Net-(J3-Pin_13) -> Net-(J3-Pin_13)
- J3 pad 16: Board_2-+BATT -> +BATT
- J3 pad 17: Board_2-Net-(J3-Pin_17) -> Net-(J3-Pin_17)
- J3 pad 18: Board_2-+BATT -> +BATT
- J3 pad 19: Board_2-Net-(J3-Pin_17) -> Net-(J3-Pin_17)
- J3 pad 2: Board_2-+BATT -> +BATT
- J3 pad 20: Board_2-+BATT -> +BATT
- J3 pad 3: Board_2-Net-(J3-Pin_1) -> Net-(J3-Pin_1)
- J3 pad 4: Board_2-+BATT -> +BATT
- J3 pad 5: Board_2-Net-(J3-Pin_5) -> Net-(J3-Pin_5)
- J3 pad 6: Board_2-+BATT -> +BATT
- J3 pad 7: Board_2-Net-(J3-Pin_5) -> Net-(J3-Pin_5)
- J3 pad 8: Board_2-+BATT -> +BATT
- J3 pad 9: Board_2-Net-(J3-Pin_11) -> Net-(J3-Pin_11)
- J3 pad 1: Board_0-Net-(J3-Pin_1) -> Net-(J3-Pin_1)
- J3 pad 10: Board_0-+BATT -> +BATT
- J3 pad 11: Board_0-Net-(J3-Pin_11) -> Net-(J3-Pin_11)
- J3 pad 12: Board_0-+BATT -> +BATT
- J3 pad 13: Board_0-Net-(J3-Pin_13) -> Net-(J3-Pin_13)
- J3 pad 14: Board_0-+BATT -> +BATT
- J3 pad 15: Board_0-Net-(J3-Pin_13) -> Net-(J3-Pin_13)
- J3 pad 16: Board_0-+BATT -> +BATT
- J3 pad 17: Board_0-Net-(J3-Pin_17) -> Net-(J3-Pin_17)
- J3 pad 18: Board_0-+BATT -> +BATT
- J3 pad 19: Board_0-Net-(J3-Pin_17) -> Net-(J3-Pin_17)
- J3 pad 2: Board_0-+BATT -> +BATT
- J3 pad 20: Board_0-+BATT -> +BATT
- J3 pad 3: Board_0-Net-(J3-Pin_1) -> Net-(J3-Pin_1)
- J3 pad 4: Board_0-+BATT -> +BATT
- J3 pad 5: Board_0-Net-(J3-Pin_5) -> Net-(J3-Pin_5)
- J3 pad 6: Board_0-+BATT -> +BATT
- J3 pad 7: Board_0-Net-(J3-Pin_5) -> Net-(J3-Pin_5)
- J3 pad 8: Board_0-+BATT -> +BATT
- J3 pad 9: Board_0-Net-(J3-Pin_11) -> Net-(J3-Pin_11)
- J3 pad 1: Board_1-Net-(J3-Pin_1) -> Net-(J3-Pin_1)
- J3 pad 10: Board_1-+BATT -> +BATT
- J3 pad 11: Board_1-Net-(J3-Pin_11) -> Net-(J3-Pin_11)
- J3 pad 12: Board_1-+BATT -> +BATT
- J3 pad 13: Board_1-Net-(J3-Pin_13) -> Net-(J3-Pin_13)
- J3 pad 14: Board_1-+BATT -> +BATT
- J3 pad 15: Board_1-Net-(J3-Pin_13) -> Net-(J3-Pin_13)
- J3 pad 16: Board_1-+BATT -> +BATT
- J3 pad 17: Board_1-Net-(J3-Pin_17) -> Net-(J3-Pin_17)
- J3 pad 18: Board_1-+BATT -> +BATT
- J3 pad 19: Board_1-Net-(J3-Pin_17) -> Net-(J3-Pin_17)
- J3 pad 2: Board_1-+BATT -> +BATT
- J3 pad 20: Board_1-+BATT -> +BATT
- J3 pad 3: Board_1-Net-(J3-Pin_1) -> Net-(J3-Pin_1)
- J3 pad 4: Board_1-+BATT -> +BATT
- J3 pad 5: Board_1-Net-(J3-Pin_5) -> Net-(J3-Pin_5)
- J3 pad 6: Board_1-+BATT -> +BATT
- J3 pad 7: Board_1-Net-(J3-Pin_5) -> Net-(J3-Pin_5)
- J3 pad 8: Board_1-+BATT -> +BATT
- J3 pad 9: Board_1-Net-(J3-Pin_11) -> Net-(J3-Pin_11)
- R10 pad 1: Board_2-ADC -> ADC
- R10 pad 2: Board_2-Net-(R10-Pad2) -> Net-(R10-Pad2)
- R10 pad 1: Board_0-ADC -> ADC
- R10 pad 2: Board_0-Net-(R10-Pad2) -> Net-(R10-Pad2)
- R10 pad 1: Board_1-ADC -> ADC
- R10 pad 2: Board_1-Net-(R10-Pad2) -> Net-(R10-Pad2)
- R10 pad 1: Board_3-ADC -> ADC
- R10 pad 2: Board_3-Net-(R10-Pad2) -> Net-(R10-Pad2)
- R11 pad 1: Board_3-Net-(R10-Pad2) -> Net-(R10-Pad2)
- R11 pad 2: Board_3-+BATT -> +BATT
- R11 pad 1: Board_2-Net-(R10-Pad2) -> Net-(R10-Pad2)
- R11 pad 2: Board_2-+BATT -> +BATT
- R11 pad 1: Board_0-Net-(R10-Pad2) -> Net-(R10-Pad2)
- R11 pad 2: Board_0-+BATT -> +BATT
- R11 pad 1: Board_1-Net-(R10-Pad2) -> Net-(R10-Pad2)
- R11 pad 2: Board_1-+BATT -> +BATT
- R2 pad 1: Board_0--BATT -> -BATT
- R2 pad 2: Board_0-Net-(R2-Pad2) -> Net-(R2-Pad2)
- R2 pad 1: Board_3--BATT -> -BATT
- R2 pad 2: Board_3-Net-(R2-Pad2) -> Net-(R2-Pad2)
- R2 pad 1: Board_1--BATT -> -BATT
- R2 pad 2: Board_1-Net-(R2-Pad2) -> Net-(R2-Pad2)
- R2 pad 1: Board_2--BATT -> -BATT
- R2 pad 2: Board_2-Net-(R2-Pad2) -> Net-(R2-Pad2)
- R4 pad 1: Board_1-D3 -> D3
- R4 pad 2: Board_1-3,3V -> 3,3V
- R4 pad 1: Board_0-D3 -> D3
- R4 pad 2: Board_0-3,3V -> 3,3V
- R4 pad 1: Board_3-D3 -> D3
- R4 pad 2: Board_3-3,3V -> 3,3V
- R4 pad 1: Board_2-D3 -> D3
- R4 pad 2: Board_2-3,3V -> 3,3V
- R5 pad 1: Board_2-D4 -> D4
- R5 pad 2: Board_2-3,3V -> 3,3V
- R5 pad 1: Board_3-D4 -> D4
- R5 pad 2: Board_3-3,3V -> 3,3V
- R5 pad 1: Board_1-D4 -> D4
- R5 pad 2: Board_1-3,3V -> 3,3V
- R5 pad 1: Board_0-D4 -> D4
- R5 pad 2: Board_0-3,3V -> 3,3V
- R6 pad 1: Board_0--BATT -> -BATT
- R6 pad 2: Board_0-D8 -> D8
- R6 pad 1: Board_3--BATT -> -BATT
- R6 pad 2: Board_3-D8 -> D8
- R6 pad 1: Board_1--BATT -> -BATT
- R6 pad 2: Board_1-D8 -> D8
- R6 pad 1: Board_2--BATT -> -BATT
- R6 pad 2: Board_2-D8 -> D8
- R8 pad 1: Board_0-/CH2 -> /CH2
- R8 pad 2: Board_0-D2 -> D2
- R8 pad 1: Board_1-/CH2 -> /CH2
- R8 pad 2: Board_1-D2 -> D2
- R8 pad 1: Board_2-/CH2 -> /CH2
- R8 pad 2: Board_2-D2 -> D2
- R8 pad 1: Board_3-/CH2 -> /CH2
- R8 pad 2: Board_3-D2 -> D2
- R9 pad 1: Board_1--BATT -> -BATT
- R9 pad 2: Board_1-ADC -> ADC
- R9 pad 1: Board_0--BATT -> -BATT
- R9 pad 2: Board_0-ADC -> ADC
- R9 pad 1: Board_2--BATT -> -BATT
- R9 pad 2: Board_2-ADC -> ADC
- R9 pad 1: Board_3--BATT -> -BATT
- R9 pad 2: Board_3-ADC -> ADC
- SW1 pad 1: Board_1-D0 -> D0
- SW1 pad 2: Board_1-Net-(R2-Pad2) -> Net-(R2-Pad2)
- SW1 pad 1: Board_2-D0 -> D0
- SW1 pad 2: Board_2-Net-(R2-Pad2) -> Net-(R2-Pad2)
- SW1 pad 1: Board_0-D0 -> D0
- SW1 pad 2: Board_0-Net-(R2-Pad2) -> Net-(R2-Pad2)
- SW1 pad 1: Board_3-D0 -> D0
- SW1 pad 2: Board_3-Net-(R2-Pad2) -> Net-(R2-Pad2)
- U2 pad 1: Board_2-D5 -> D5
- U2 pad 10: Board_2-Net-(J3-Pin_1) -> Net-(J3-Pin_1)
- U2 pad 11: Board_2-Net-(J3-Pin_1) -> Net-(J3-Pin_1)
- U2 pad 12: Board_2-Net-(J3-Pin_5) -> Net-(J3-Pin_5)
- U2 pad 13: Board_2-Net-(J3-Pin_5) -> Net-(J3-Pin_5)
- U2 pad 14: Board_2-Net-(J3-Pin_11) -> Net-(J3-Pin_11)
- U2 pad 15: Board_2-Net-(J3-Pin_13) -> Net-(J3-Pin_13)
- U2 pad 16: Board_2-Net-(J3-Pin_17) -> Net-(J3-Pin_17)
- U2 pad 2: Board_2-D6 -> D6
- U2 pad 3: Board_2-D7 -> D7
- U2 pad 4: Board_2-TX -> D8
- U2 pad 5: Board_2-TX -> D8
- U2 pad 6: Board_2-RX -> RX
- U2 pad 7: Board_2-RX -> RX
- U2 pad 8: Board_2--BATT -> -BATT
- U2 pad 9: Board_2-+BATT -> +BATT
- U2 pad 1: Board_1-D5 -> D5
- U2 pad 10: Board_1-Net-(J3-Pin_1) -> Net-(J3-Pin_1)
- U2 pad 11: Board_1-Net-(J3-Pin_1) -> Net-(J3-Pin_1)
- U2 pad 12: Board_1-Net-(J3-Pin_5) -> Net-(J3-Pin_5)
- U2 pad 13: Board_1-Net-(J3-Pin_5) -> Net-(J3-Pin_5)
- U2 pad 14: Board_1-Net-(J3-Pin_11) -> Net-(J3-Pin_11)
- U2 pad 15: Board_1-Net-(J3-Pin_13) -> Net-(J3-Pin_13)
- U2 pad 16: Board_1-Net-(J3-Pin_17) -> Net-(J3-Pin_17)
- U2 pad 2: Board_1-D6 -> D6
- U2 pad 3: Board_1-D7 -> D7
- U2 pad 4: Board_1-TX -> D8
- U2 pad 5: Board_1-TX -> D8
- U2 pad 6: Board_1-RX -> RX
- U2 pad 7: Board_1-RX -> RX
- U2 pad 8: Board_1--BATT -> -BATT
- U2 pad 9: Board_1-+BATT -> +BATT
- U2 pad 1: Board_0-D5 -> D5
- U2 pad 10: Board_0-Net-(J3-Pin_1) -> Net-(J3-Pin_1)
- U2 pad 11: Board_0-Net-(J3-Pin_1) -> Net-(J3-Pin_1)
- U2 pad 12: Board_0-Net-(J3-Pin_5) -> Net-(J3-Pin_5)
- U2 pad 13: Board_0-Net-(J3-Pin_5) -> Net-(J3-Pin_5)
- U2 pad 14: Board_0-Net-(J3-Pin_11) -> Net-(J3-Pin_11)
- U2 pad 15: Board_0-Net-(J3-Pin_13) -> Net-(J3-Pin_13)
- U2 pad 16: Board_0-Net-(J3-Pin_17) -> Net-(J3-Pin_17)
- U2 pad 2: Board_0-D6 -> D6
- U2 pad 3: Board_0-D7 -> D7
- U2 pad 4: Board_0-TX -> D8
- U2 pad 5: Board_0-TX -> D8
- U2 pad 6: Board_0-RX -> RX
- U2 pad 7: Board_0-RX -> RX
- U2 pad 8: Board_0--BATT -> -BATT
- U2 pad 9: Board_0-+BATT -> +BATT
- U2 pad 1: Board_3-D5 -> D5
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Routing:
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- added copper zone on B.Cu, net -BATT
- added copper zone on F.Cu, net -BATT
- removed copper zone on B.Cu, net Board_0--BATT
- removed copper zone on F.Cu, net Board_0--BATT
- removed copper zone on B.Cu, net Board_1--BATT
- removed copper zone on F.Cu, net Board_1--BATT
- removed copper zone on B.Cu, net Board_2--BATT
- removed copper zone on F.Cu, net Board_2--BATT
- removed copper zone on B.Cu, net Board_3--BATT
- removed copper zone on F.Cu, net Board_3--BATT
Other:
- outline, holes or cut-outs redrawn
- board text added: "AP: 1.2.3.4"
- board text added: "sLiachdDingens V2.1"
- board text removed: "AP:1.2.3.4"
- board text removed: "sLiachdDingens V2"
